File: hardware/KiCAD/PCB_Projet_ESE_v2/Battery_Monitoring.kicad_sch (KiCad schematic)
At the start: 73 parts, among them U16 MCP1802x-xx02xOT

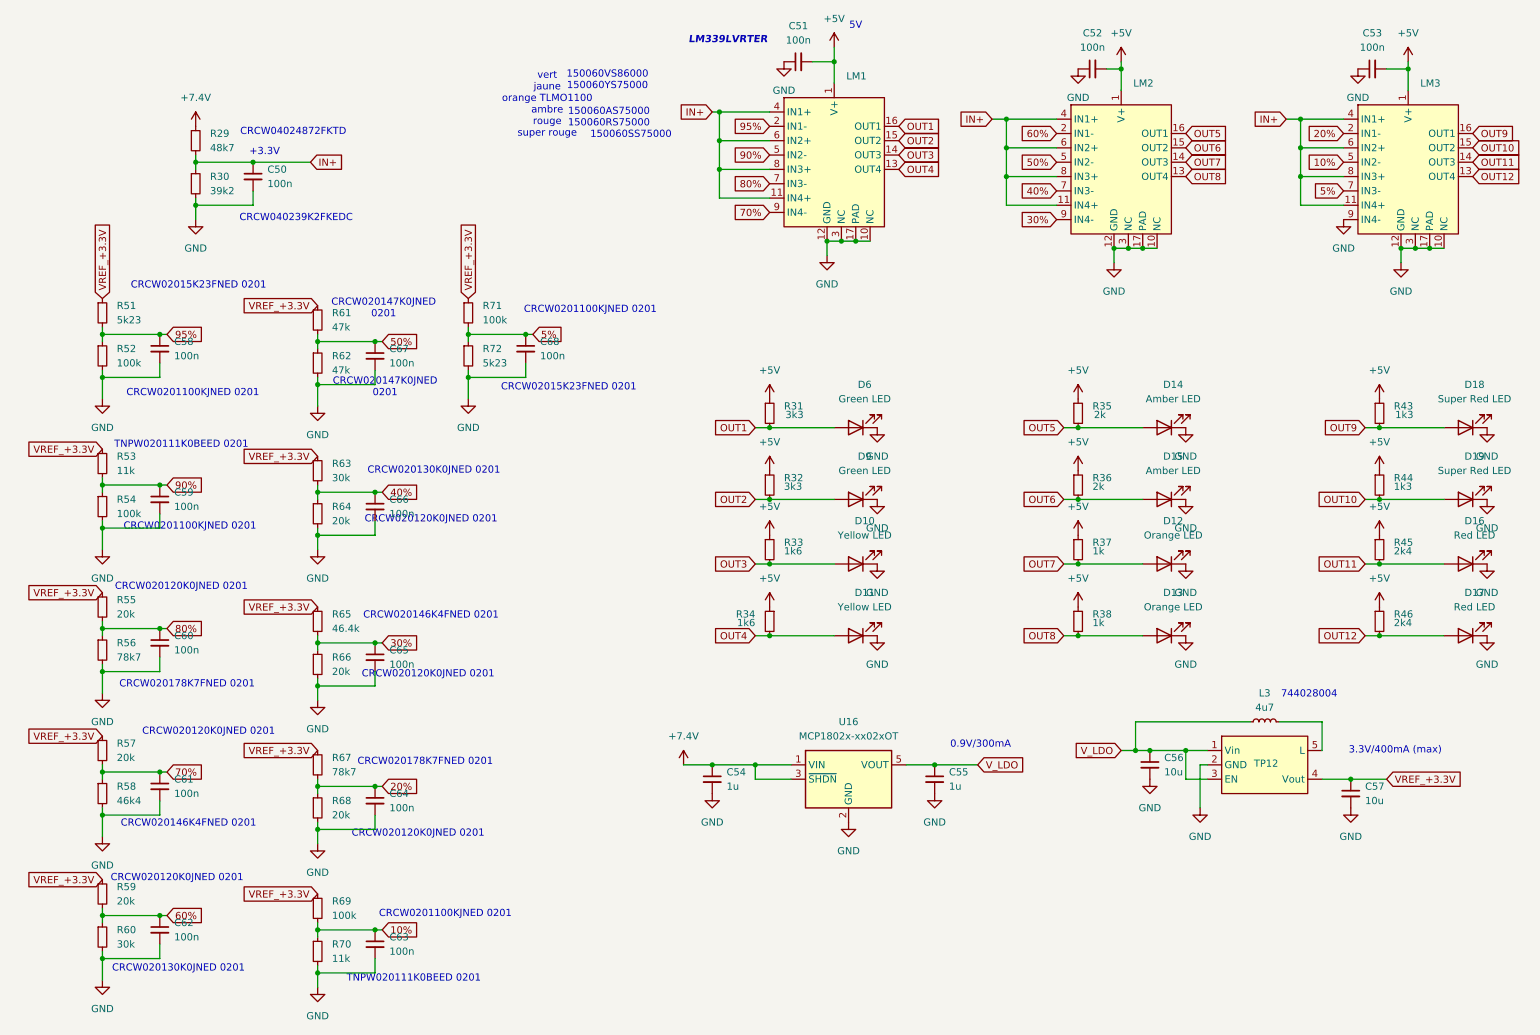
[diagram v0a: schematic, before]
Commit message: Finish README
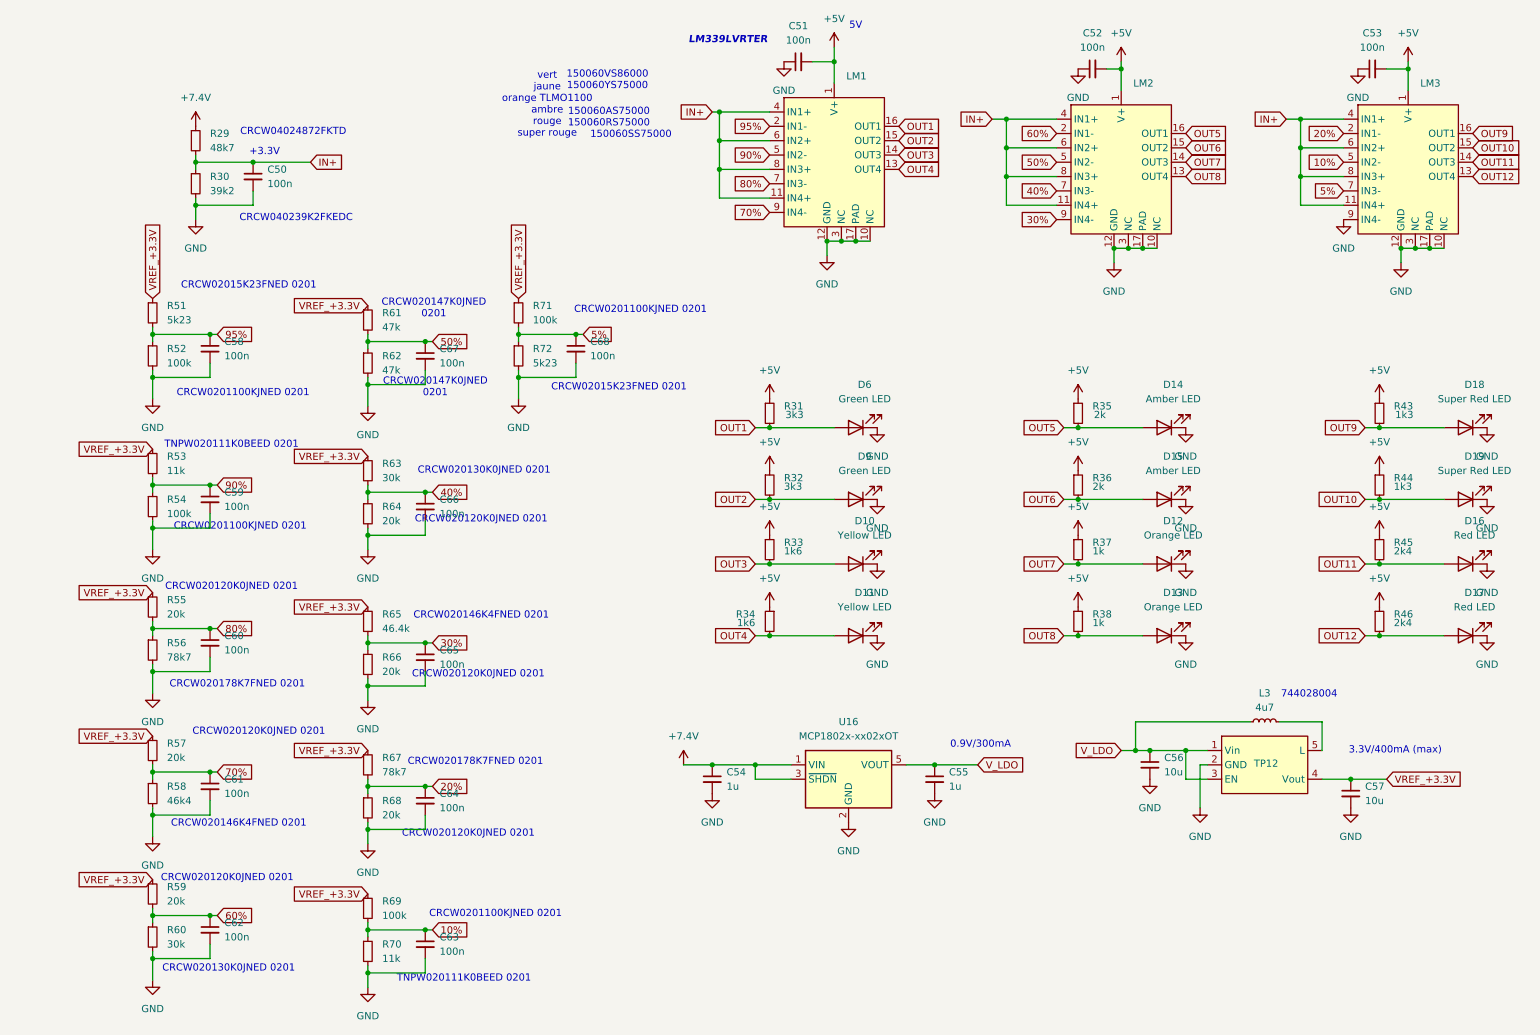
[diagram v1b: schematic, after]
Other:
- moved on the sheet: C58, C59, C60, C61, C62, C63, C64, C65, C66, C67, C68, R51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
